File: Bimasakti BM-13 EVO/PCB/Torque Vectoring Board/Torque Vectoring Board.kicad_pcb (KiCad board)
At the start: 2 copper layers, 72.8 x 82.8 mm, 23 parts, among them U3 SN65HVD230, U4 SN65HVD230, U5 ADS1115IDGS

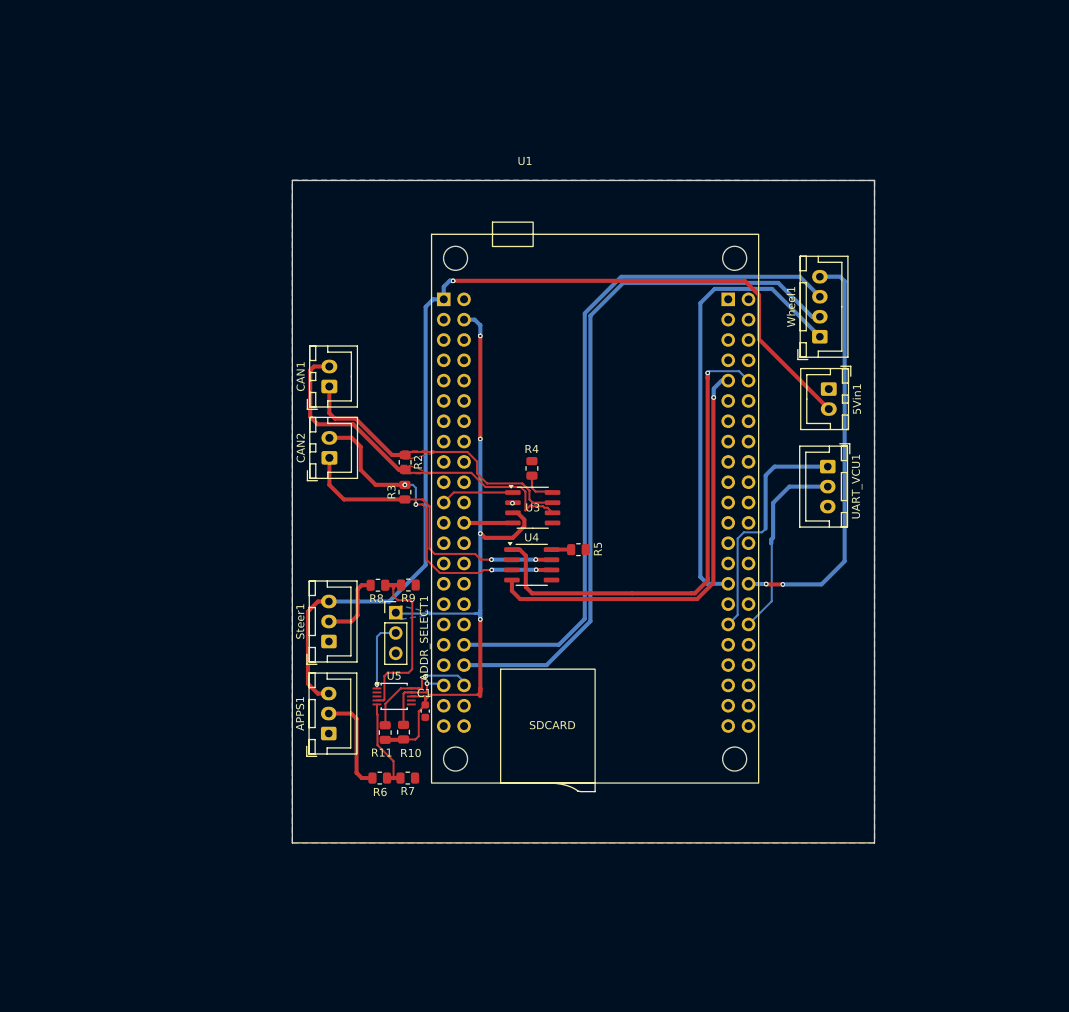
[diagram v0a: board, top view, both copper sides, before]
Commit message: cicil assembly
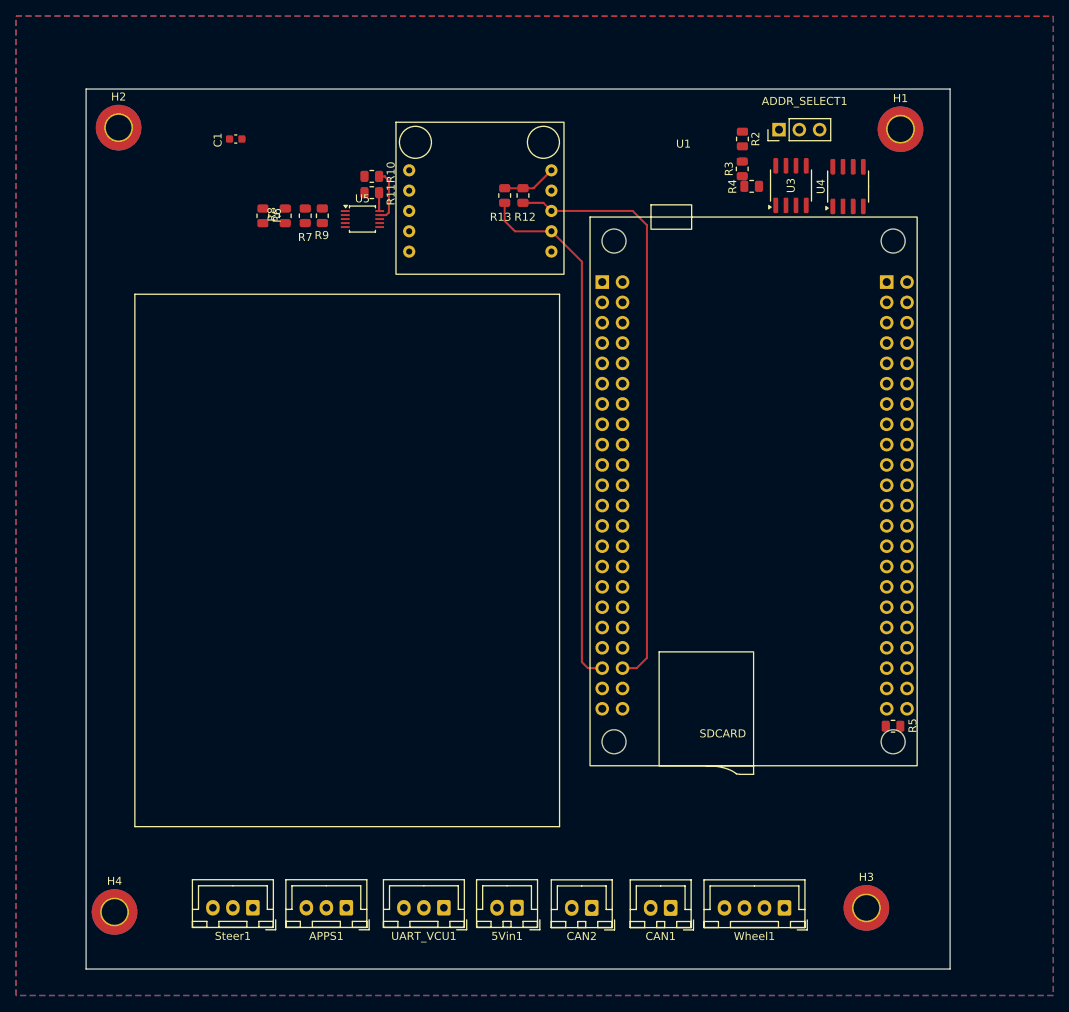
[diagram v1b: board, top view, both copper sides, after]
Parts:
- added H1: MountingHole_Pad, MountingHole:MountingHole_3.2mm_M3_ISO7380_Pad_TopBottom, F.Cu at (146.5, 34.2)
- added H2: MountingHole_Pad, MountingHole:MountingHole_3.2mm_M3_ISO7380_Pad_TopBottom, F.Cu at (48.8, 34.0)
- added H3: MountingHole_Pad, MountingHole:MountingHole_3.2mm_M3_ISO7380_Pad_TopBottom, F.Cu at (142.2, 131.6)
- added H4: MountingHole_Pad, MountingHole:MountingHole_3.2mm_M3_ISO7380_Pad_TopBottom, F.Cu at (48.3, 132.1)
- added R12: 10K, Resistor_SMD:R_0805_2012Metric, F.Cu at (99.3, 42.5)
- added R13: 10K, Resistor_SMD:R_0805_2012Metric, F.Cu at (97.0, 42.5)
- added U2: ~, 0_bno055:0_BNO055, F.Cu at (94.9, 25.9)
- moved CAN1 77.9 mm to (117.8, 131.6), turned to 180 degrees
- moved ADDR_SELECT1 77.1 mm to (131.3, 34.3), turned to 90 degrees
- moved 5Vin1 75.6 mm to (98.6, 131.6), turned to 180 degrees
- moved C1 75.3 mm to (63.4, 35.5), turned to 180 degrees
- moved UART_VCU1 73.1 mm to (89.4, 131.6), turned to 180 degrees
- moved R6 71.8 mm to (66.8, 45.1), turned to 90 degrees
- moved Wheel1 71.5 mm to (132.0, 131.6), turned to 180 degrees
- moved R7 71.4 mm to (72.1, 45.1), turned to -90 degrees
- moved R10 69.6 mm to (80.4, 40.1), turned to 0 degrees
- moved R11 67.5 mm to (80.4, 42.2), turned to 0 degrees
- moved CAN2 65.1 mm to (107.9, 131.6), turned to 180 degrees
- moved U4 61.6 mm to (140.0, 41.4), turned to 90 degrees
- moved U5 59.8 mm to (79.2, 45.5)
- moved R2 58.4 mm to (126.7, 35.5)
- moved R3 58.4 mm to (126.7, 39.2)
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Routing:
- net 5V: track 124.1 -> 0.00 mm, vias 1 -> 0
- net MISO: track 88.4 -> 0.00 mm
- net MOSI: track 86.9 -> 0.00 mm
- net 3V3: track 90.6 -> 6.77 mm, vias 4 -> 0
- net SDA: track 10.2 -> 73.7 mm, vias 1 -> 0
- net CAN2_TX: track 61.7 -> 0.00 mm, vias 1 -> 0
- net SCL: track 16.5 -> 76.7 mm, vias 1 -> 0
- net SCK: track 56.2 -> 0.00 mm
- net CAN2_RX: track 54.4 -> 0.00 mm, vias 1 -> 0
- net SS: track 51.6 -> 0.00 mm, vias 2 -> 0
- net CANL1: track 45.6 -> 0.00 mm
- net CANL2: track 41.6 -> 0.00 mm, vias 4 -> 0
- net CANH2: track 38.1 -> 0.00 mm, vias 2 -> 0
- net CANH1: track 37.7 -> 0.00 mm
- net TX1: track 30.1 -> 0.00 mm
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- removed copper zone on B.Cu, net 3V3
- removed copper zone on F.Cu, net CANH1
- removed copper zone on F.Cu, net CANL1
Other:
- board size 72.8 x 82.8 mm -> 108 x 110 mm
